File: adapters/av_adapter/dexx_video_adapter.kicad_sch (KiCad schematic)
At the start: 6 parts, among them J1 SCART-F, J2 Pr, J3 Y, J4 Pb, J5 AudioJack3, J6 DB15_Female_HighDensity

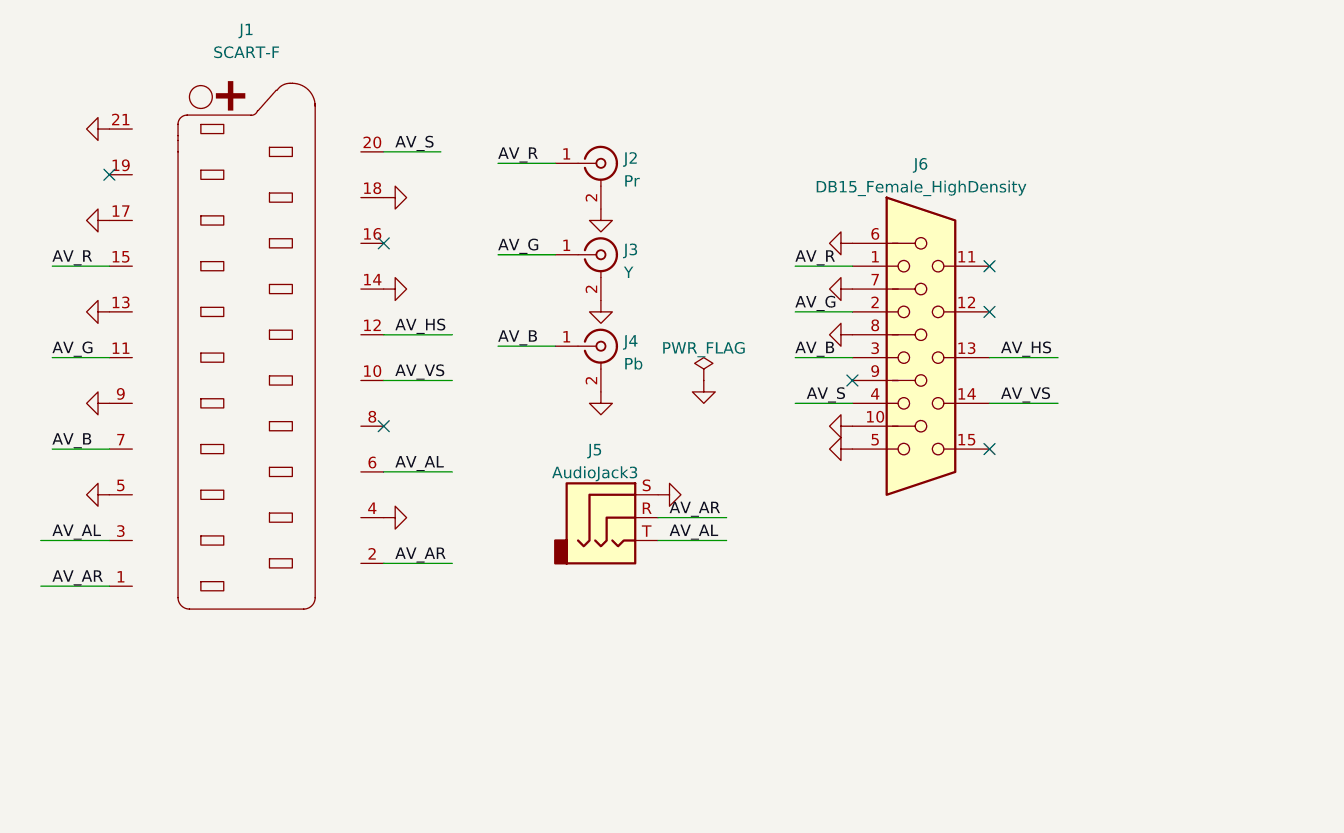
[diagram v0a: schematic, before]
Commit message: update av_adapter board to v1.1
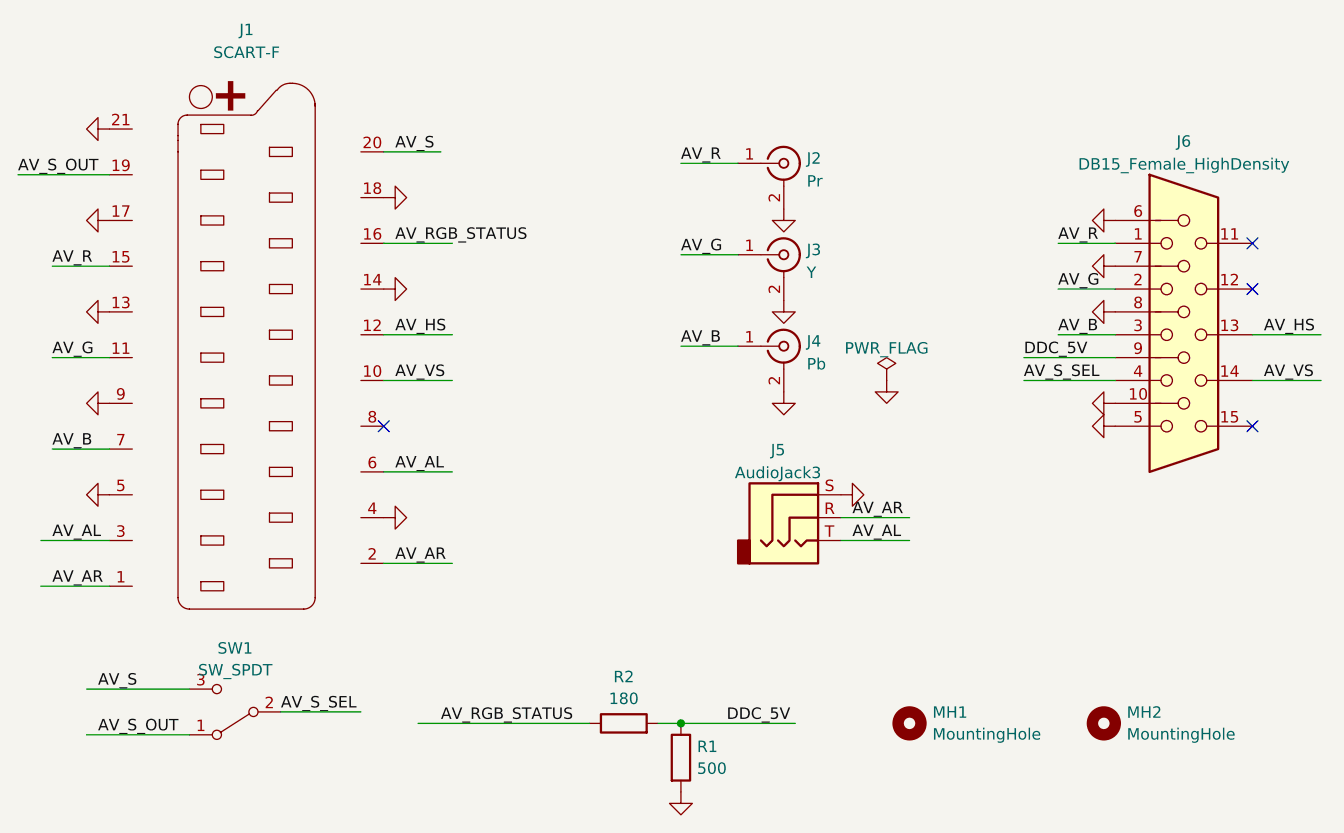
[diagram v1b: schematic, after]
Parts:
- added MH1, MH2: MountingHole, MountingHole:MountingHole_3.2mm_M3_ISO14580_Pad, symbol Mechanical:MountingHole
- added R1: 500, custom_components:SM0603_Resistor_libcms, symbol Device:R
- added R2: 180, custom_components:SM0603_Resistor_libcms, symbol Device:R
- added SW1: SW_SPDT, custom_components:SWITCH_11MA1QS1, symbol Switch:SW_SPDT
- J5: footprint custom_components:SJ1-3533NG -> Connector_Audio:Jack_3.5mm_CUI_SJ1-3533NG_Horizontal
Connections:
- net AV_S: now also SW1.3 (C); no longer J6.4
- net GND: now also R1.2
- net AV_RGB_STATUS: now reaches J1.16 (P16)
- net AV_RGB_STATUS: now also R2.1
- net AV_S_OUT: now reaches J1.19 (P19)
- net AV_S_OUT: now also SW1.1 (A)
- net DDC_5V: now reaches J6.9
- net DDC_5V: now also R1.1, R2.2
- new net AV_S_SEL: J6.4, SW1.2 (B)
- no-connect marks 7 -> 4
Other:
- title: DExx AV adapter -> AV adapter
- moved on the sheet: J2, J3, J4, J5, J6
